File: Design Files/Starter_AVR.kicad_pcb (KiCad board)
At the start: 2 copper layers, 90.5 x 67.5 mm, 48 parts, among them CON1 USB-MICRO-B, IC1 ATMEGA32-P, J2 SIL8, J3 SIL8, J4 SIL8, J5 SIL8, K1 BARREL, K2 CONN_3, K3 CONN_3, K4 CONN_3, P1 CONN_1, P2 CONN_1, P3 CONN_1, P4 CONN_1, P6 CONN_5X2, SW1 rst, SW2 SPST, SW3 SPST, SW4 SPST, U1 CP2102, U2 LM317S, X1 16Mhz

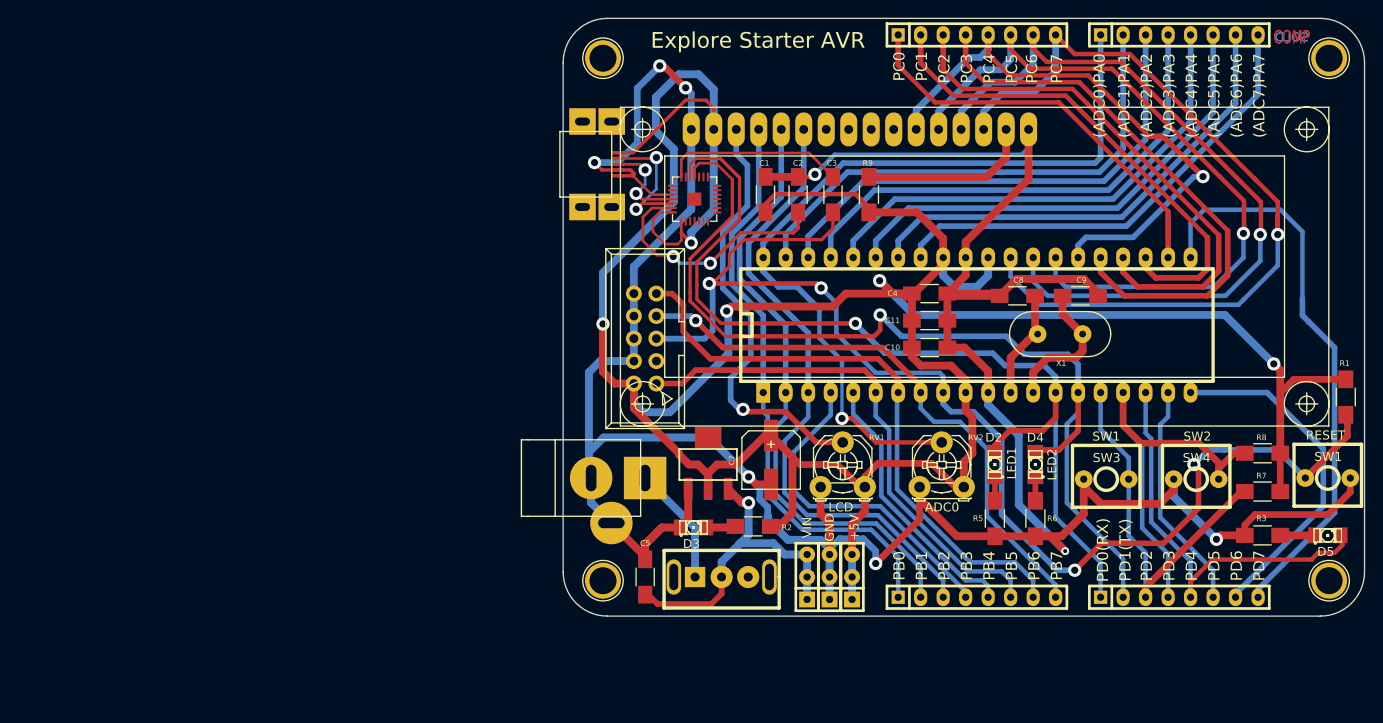
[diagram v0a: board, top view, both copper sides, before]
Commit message: new design
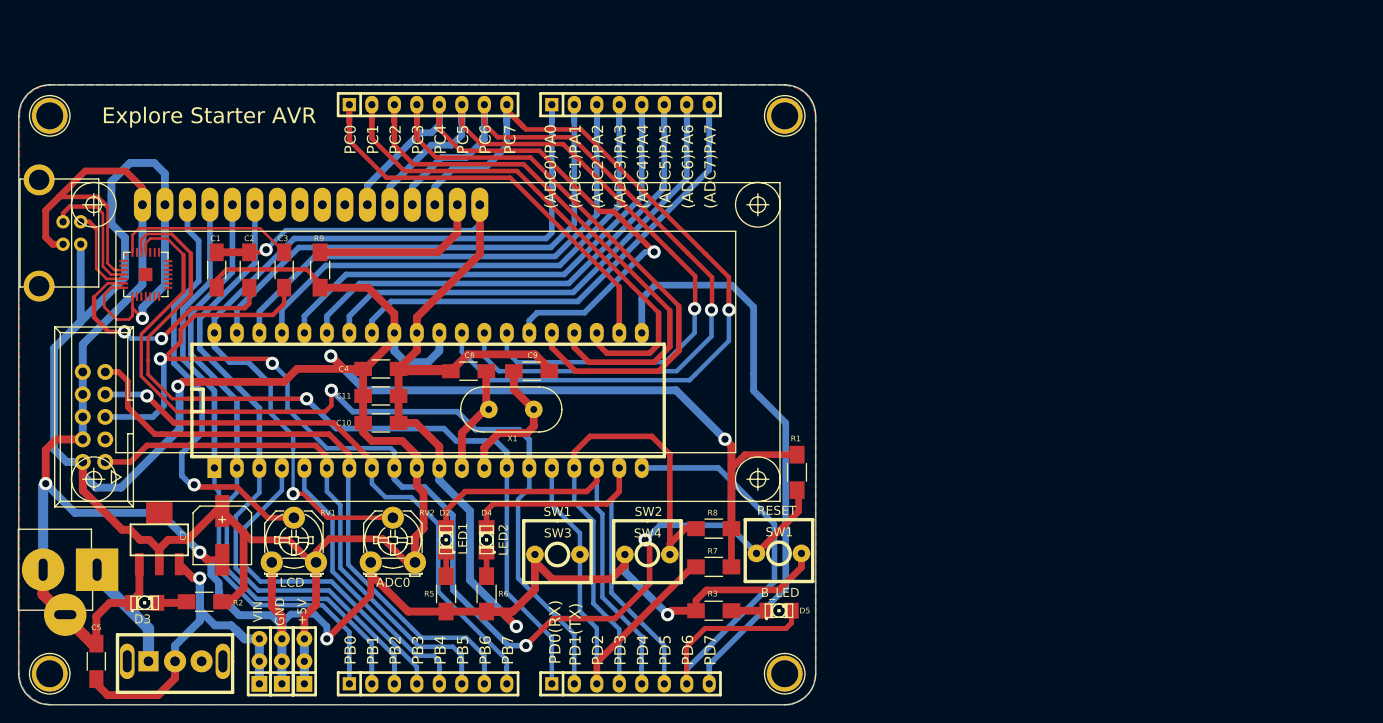
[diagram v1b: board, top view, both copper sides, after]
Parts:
- removed LOGO: , lOGO:LOGO (1)
- CON1: footprint EE:USB_Micro-B_SMD_NEW -> Connect:USB_B
- K1: footprint Connect:JACK_ALIM -> EE:DC_Jack
- LCD1: footprint lcd_2x16_led_backlight-HY-1602F -> EE:lcd_2x16_led_backlight-HY-1602F
- SW2: footprint EE:SPSPT_XL_NEW -> EE:SlideSwitch_Big
- moved P1 63.4 mm to (44.5, 111.5)
- moved P6 62.9 mm to (49.5, 82.5)
- moved P2 62.8 mm to (44.5, 48.5)
- moved K1 62.7 mm to (43.8, 99.8)
- moved J5 62.7 mm to (110.1, 112.6)
- moved J3 62.7 mm to (87.2, 112.6)
- moved C5 62.7 mm to (49.8, 110.1)
- moved K4 62.6 mm to (68.2, 110.1)
- moved K2 62.6 mm to (73.3, 110.1)
- moved K3 62.6 mm to (70.7, 110.1)
- moved C2 62.6 mm to (67.1, 65.9)
- moved D4 62.6 mm to (93.9, 96.4)
- moved R6 62.6 mm to (93.9, 102.5)
- moved SW3 62.6 mm to (101.9, 98.0)
- moved SW4 62.6 mm to (112.0, 98.0)
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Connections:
- D2 pad 1: /rxd -> /L1
- D4 pad 1: /txd -> /L2
- IC1 pad 18: /BL -> /L1
- IC1 pad 19: Net-(IC1-Pad19) -> /L2
- IC1 pad 20: Net-(IC1-Pad20) -> /BL
- J5 pad 5: /BL -> /L1
- J5 pad 6: Net-(IC1-Pad19) -> /L2
- J5 pad 7: Net-(IC1-Pad20) -> /BL
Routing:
- net /L1: track 0.00 -> 49.4 mm
- net /L2: track 0.00 -> 48.0 mm
- net /BL: track 46.9 -> 89.7 mm
- net Net-(IC1-Pad20): track 38.5 -> 0.00 mm
- net Net-(IC1-Pad19): track 26.0 -> 0.00 mm
- net GND: track 371.5 -> 389.6 mm, vias 8 -> 6
- net /rxd: track 107.6 -> 97.4 mm
- net /DC IN: track 37.2 -> 46.0 mm
- net /txd: track 111.2 -> 102.5 mm
- net /S2: track 48.2 -> 56.8 mm
- net Net-(CON1-Pad2): track 15.7 -> 10.2 mm, vias 2 -> 0
- net /D7: track 95.2 -> 100.4 mm
- net /rst: track 153.0 -> 148.2 mm
- net Net-(CON1-Pad3): track 10.8 -> 14.8 mm, vias 2 -> 0
- net /D5: track 83.0 -> 86.8 mm
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- added copper zone on F.Cu, net /+5V
- added copper zone on B.Cu, net GND
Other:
- board size 90.5 x 67.5 mm -> 90 x 70 mm
- net class Default: clearance 0.1778 -> 0.254
- rule trace_clearance: 0.1778 -> 0.254
- board text added: "B_LED"
- board text added: "LCD Connection D0-D4->PC4-PC7 RS->PB0 R/W->PB1 EN->PB2 LED1->PD4 LED2->PD5 SW1->PD2 SW2->PD3"
- board text removed: "COMP"
- board text removed: "LCD Connection D0-D4->PC4-PC7 RS->PB0 R/W->PB1 E->PB2 LED1->PD0 LED2->PD1 SW1->PD2 SW2->PD3"
- board text removed: "SOLD"

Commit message: LCD connection Legend
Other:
- board text added: "LCD Connection D4-D7->PC4-PC7 RS->PB0 R/W->PB1 EN->PB2 LED1->PD4 LED2->PD5 SW1->PD2 SW2->PD3"
- board text removed: "LCD Connection D0-D4->PC4-PC7 RS->PB0 R/W->PB1 EN->PB2 LED1->PD4 LED2->PD5 SW1->PD2 SW2->PD3"
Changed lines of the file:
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@@
-(kicad_pcb (version 4) (host pcbnew "(2015-01-16 BZR 5376)-product")
+(kicad_pcb (version 4) (host pcbnew 4.0.5)
   (general
     (links 132)
     (no_connects 0)
-    (area 40.948999 44.933999 131.099001 115.084001)
+    (area 32.494999 44.933999 132.334 115.084001)
     (thickness 1.6)
     (drawings 55)
@@
     (effects (font (size 2.54 2.54) (thickness 0.508)) (justify mirror))
   )
-  (gr_text "LCD Connection\nD0-D4->PC4-PC7\nRS->PB0\nR/W->PB1\nEN->PB2\n\nLED1->PD4\nLED2->PD5\n\nSW1->PD2\nSW2->PD3" (at 118.11 60.579) (layer B.SilkS)
+  (gr_text "LCD Connection\nD4-D7->PC4-PC7\nRS->PB0\nR/W->PB1\nEN->PB2\n\nLED1->PD4\nLED2->PD5\n\nSW1->PD2\nSW2->PD3" (at 118.11 60.579) (layer B.SilkS)
     (effects (font (size 1.016 1.016) (thickness 0.254) italic) (justify left mirror))
   )
